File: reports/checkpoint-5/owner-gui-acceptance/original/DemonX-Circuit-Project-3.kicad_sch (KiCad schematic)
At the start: 3 parts, among them J1 5V INPUT

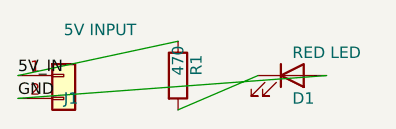
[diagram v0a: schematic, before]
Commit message: Package exact KiCad owner GUI acceptance fixture
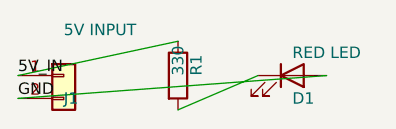
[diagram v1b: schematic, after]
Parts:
- R1: value 470 -> 330
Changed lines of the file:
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@@
 (kicad_sch
-	(version 20250114)
+	(version 20260306)
 	(generator "eeschema")
-	(generator_version "9.0")
+	(generator_version "10.0")
 	(paper "A4")
 	(title_block
 		(title "DX_LED_Smoke")
+	)
+	(wire
+		(pts
+			(xy 80.01 50.8) (xy 45.72 53.34)
+		)
+		(stroke
+			(width 0)
+			(type default)
+		)
+	)
+	(wire
+		(pts
+			(xy 63.5 54.61) (xy 72.39 50.8)
+		)
+		(stroke
+			(width 0)
+			(type default)
+		)
+	)
+	(wire
+		(pts
+			(xy 45.72 50.8) (xy 63.5 46.99)
+		)
+		(stroke
+			(width 0)
+			(type default)
+		)
+	)
+	(label "GND"
+		(at 45.72 53.34 0)
+		(effects
+			(font
+				(size 1.27 1.27)
+			)
+			(justify left bottom)
+		)
+	)
+	(label "5V_IN"
+		(at 45.72 50.8 0)
+		(effects
+			(font
+				(size 1.27 1.27)
+			)
+			(justify left bottom)
+		)
+	)
+	(symbol
+		(lib_id "Device:LED")
+		(at 76.2 50.8 0)
+		(unit 1)
+		(body_style 1)
+		(exclude_from_sim no)
+		(in_bom yes)
+		(on_board yes)
+		(in_pos_files yes)
+		(dnp no)
+		(property "Reference" "D1"
+			(at 76.2 53.34 0)
+			(show_name no)
+			(do_not_autoplace no)
+			(effects
+				(font
+					(size 1.27 1.27)
+				)
+				(justify left)
+			)
+		)
+		(property "Value" "RED LED"
+			(at 76.2 48.26 0)
+			(show_name no)
+			(do_not_autoplace no)
+			(effects
+				(font
+					(size 1.27 1.27)
+				)
+				(justify left)
+			)
+		)
+		(property "Footprint" "LED_THT:LED_D5.0mm"
+			(at 76.2 50.8 0)
+			(hide yes)
+			(show_name no)
+			(do_not_autoplace no)
+			(effects
+				(font
+					(size 1.27 1.27)
+				)
+			)
+		)
+		(property "Datasheet" ""
+			(at 76.2 50.8 0)
+			(show_name no)
+			(do_not_autoplace no)
+			(effects
+				(font
+					(size 1.27 1.27)
+				)
+			)
+		)
+		(property "Description" ""
+			(at 76.2 50.8 0)
+			(show_name no)
+			(do_not_autoplace no)
+			(effects
+				(font
+					(size 1.27 1.27)
+				)
+			)
+		)
+		(pin "1"
+		)
+		(pin "2"
+		)
+		(instances
+			(project "DX_LED_Smoke"
+				(path "/610e112a-8e5a-4db8-8fc4-4b25843f46d9"
+					(reference "D1")
+					(unit 1)
+				)
+			)
+		)
+	)
+	(symbol
+		(lib_id "Device:R")
+		(at 63.5 50.8 0)
+		(unit 1)
+		(body_style 1)
+		(exclude_from_sim no)
+		(in_bom yes)
+		(on_board yes)
+		(in_pos_files yes)
+		(dnp no)
+		(property "Reference" "R1"
+			(at 65.532 50.8 90)
+			(show_name no)
+			(do_not_autoplace no)
+			(effects
+				(font
+					(size 1.27 1.27)
+				)
+				(justify left)
+			)
+		)
+		(property "Value" "330"
+			(at 63.5 50.8 90)
+			(show_name no)
+			(do_not_autoplace no)
+			(effects
+				(font
+					(size 1.27 1.27)
+				)
+				(justify left)
+			)
+		)
+		(property "Footprint" "Resistor_THT:R_Axial_DIN0207_L6.3mm_D2.5mm_P7.62mm_Horizontal"
+			(at 61.722 50.8 90)
+			(hide yes)
+			(show_name no)
+			(do_not_autoplace no)
+			(effects
+				(font
+					(size 1.27 1.27)
+				)
+			)
+		)
+		(property "Datasheet" ""
+			(at 63.5 50.8 0)
+			(show_name no)
+			(do_not_autoplace no)
+			(effects
+				(font
+					(size 1.27 1.27)
+				)
+			)
+		)
+		(property "Description" ""
+			(at 63.5 50.8 0)
+			(show_name no)
+			(do_not_autoplace no)
+			(effects
+				(font
+					(size 1.27 1.27)
+				)
+			)
+		)
+		(pin "1"
+		)
+		(pin "2"
+		)
+		(instances
+			(project "DX_LED_Smoke"
+				(path "/610e112a-8e5a-4db8-8fc4-4b25843f46d9"
+					(reference "R1")
+					(unit 1)
+				)
+			)
+		)
 	)
 	(symbol
@@
 		(at 50.8 50.8 0)
 		(unit 1)
+		(body_style 1)
 		(exclude_from_sim no)
 		(in_bom yes)
 		(on_board yes)
+		(in_pos_files yes)
 		(dnp no)
-		(fields_autoplaced no)
 		(property "Reference" "J1"
-			(at 50.8 53.34 0.0000)
+			(at 50.8 53.34 0)
+			(show_name no)
+			(do_not_autoplace no)
 			(effects
 				(font
@@
 		)
 		(property "Value" "5V INPUT"
-			(at 50.8 45.72 0.0000)
+			(at 50.8 45.72 0)
+			(show_name no)
+			(do_not_autoplace no)
 			(effects
 				(font
@@
 		)
 		(property "Footprint" "Connector_PinHeader_2.54mm:PinHeader_1x02_P2.54mm_Vertical"
-			(at 50.8 50.8 0.0000)
-			(effects
-				(font
-					(size 1.27 1.27)
-				)
-				(hide yes)
+			(at 50.8 50.8 0)
+			(hide yes)
+			(show_name no)
+			(do_not_autoplace no)
+			(effects
+				(font
+					(size 1.27 1.27)
+				)
+			)
+		)
+		(property "Datasheet" ""
+			(at 50.8 50.8 0)
+			(show_name no)
+			(do_not_autoplace no)
+			(effects
+				(font
+					(size 1.27 1.27)
+				)
+			)
+		)
+		(property "Description" ""
+			(at 50.8 50.8 0)
+			(show_name no)
+			(do_not_autoplace no)
+			(effects
+				(font
+					(size 1.27 1.27)
+				)
 			)
 		)
@@
 		(instances
 			(project "DX_LED_Smoke"
-				(path "/a2993e05-0265-4943-949c-8fffc8eec7bd"
+				(path "/610e112a-8e5a-4db8-8fc4-4b25843f46d9"
 					(reference "J1")
 					(unit 1)
 				)
 			)
-		)
-	)
-	(symbol
-		(lib_id "Device:R")
-		(at 63.5 50.8 0)
-		(unit 1)
-		(exclude_from_sim no)
-		(in_bom yes)
-		(on_board yes)
-		(dnp no)
-		(fields_autoplaced no)
-		(property "Reference" "R1"
-			(at 65.532 50.8 90)
-			(effects
-				(font
-					(size 1.27 1.27)
-				)
-				(justify left)
-			)
-		)
-		(property "Value" "470"
-			(at 63.5 50.8 90)
-			(effects
-				(font
-					(size 1.27 1.27)
-				)
-				(justify left)
-			)
-		)
-		(property "Footprint" "Resistor_THT:R_Axial_DIN0207_L6.3mm_D2.5mm_P7.62mm_Horizontal"
-			(at 61.722 50.8 90)
-			(effects
-				(font
-					(size 1.27 1.27)
-				)
-				(hide yes)
-			)
-		)
-		(pin "1"
-		)
-		(pin "2"
-		)
-		(instances
-			(project "DX_LED_Smoke"
-				(path "/a2993e05-0265-4943-949c-8fffc8eec7bd"
-					(reference "R1")
-					(unit 1)
-				)
-			)
-		)
-	)
-	(symbol
-		(lib_id "Device:LED")
-		(at 76.2 50.8 0)
-		(unit 1)
-		(exclude_from_sim no)
-		(in_bom yes)
-		(on_board yes)
-		(dnp no)
-		(fields_autoplaced no)
-		(property "Reference" "D1"
-			(at 76.2 53.34 0.0000)
-			(effects
-				(font
-					(size 1.27 1.27)
-				)
-				(justify left)
-			)
-		)
-		(property "Value" "RED LED"
-			(at 76.2 48.26 0.0000)
-			(effects
-				(font
-					(size 1.27 1.27)
-				)
-				(justify left)
-			)
-		)
-		(property "Footprint" "LED_THT:LED_D5.0mm"
-			(at 76.2 50.8 0.0000)
-			(effects
-				(font
-					(size 1.27 1.27)
-				)
-				(hide yes)
-			)
-		)
-		(pin "1"
-		)
-		(pin "2"
-		)
-		(instances
-			(project "DX_LED_Smoke"
-				(path "/a2993e05-0265-4943-949c-8fffc8eec7bd"
-					(reference "D1")
-					(unit 1)
-				)
-			)
-		)
-	)
-	(wire
-		(pts
-			(xy 45.72 50.8) (xy 63.5 46.99)
-		)
-		(stroke
-			(width 0)
-			(type default)
-		)
-	)
-	(wire
-		(pts
-			(xy 63.5 54.61) (xy 72.39 50.8)
-		)
-		(stroke
-			(width 0)
-			(type default)
-		)
-	)
-	(wire
-		(pts
-			(xy 80.01 50.8) (xy 45.72 53.34)
-		)
-		(stroke
-			(width 0)
-			(type default)
-		)
-	)
-	(label "5V_IN"
-		(at 45.72 50.8 0.0000)
-		(effects
-			(font
-				(size 1.27 1.27)
-			)
-			(justify left bottom)
-		)
-	)
-	(label "GND"
-		(at 45.72 53.34 0.0000)
-		(effects
-			(font
-				(size 1.27 1.27)
-			)
-			(justify left bottom)
 		)
 	)
@@
 		)
 	)
-	(embedded_fonts no)
 )
